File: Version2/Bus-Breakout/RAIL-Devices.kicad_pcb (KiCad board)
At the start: 2 copper layers, 99.8 x 19.5 mm, 33 parts, among them J2 Conn_01x30_Pin, J5 Conn_02x30_Odd_Even, P1 Jumper4x1, P10 Jumper4x1, P11 Jumper4x1, P12 Jumper4x1, P13 Jumper4x1, P14 Jumper4x1, P15 Jumper4x1, P16 Jumper4x1, P17 Jumper4x1, P18 Jumper4x1, P19 Jumper4x1, P2 Jumper4x1, P20 Jumper4x1, P21 Jumper4x1, P22 Jumper4x1, P23 Jumper4x1, P24 Jumper4x1, P25 Jumper4x1, P26 Jumper4x1, P27 Jumper4x1, P28 Jumper4x1, P29 Jumper4x1, P3 Jumper4x1, P30 Jumper4x1, P4 Jumper4x1, P5 Jumper4x1, P6 Jumper4x1, P7 Jumper4x1, P8 Jumper4x1, P9 Jumper4x1

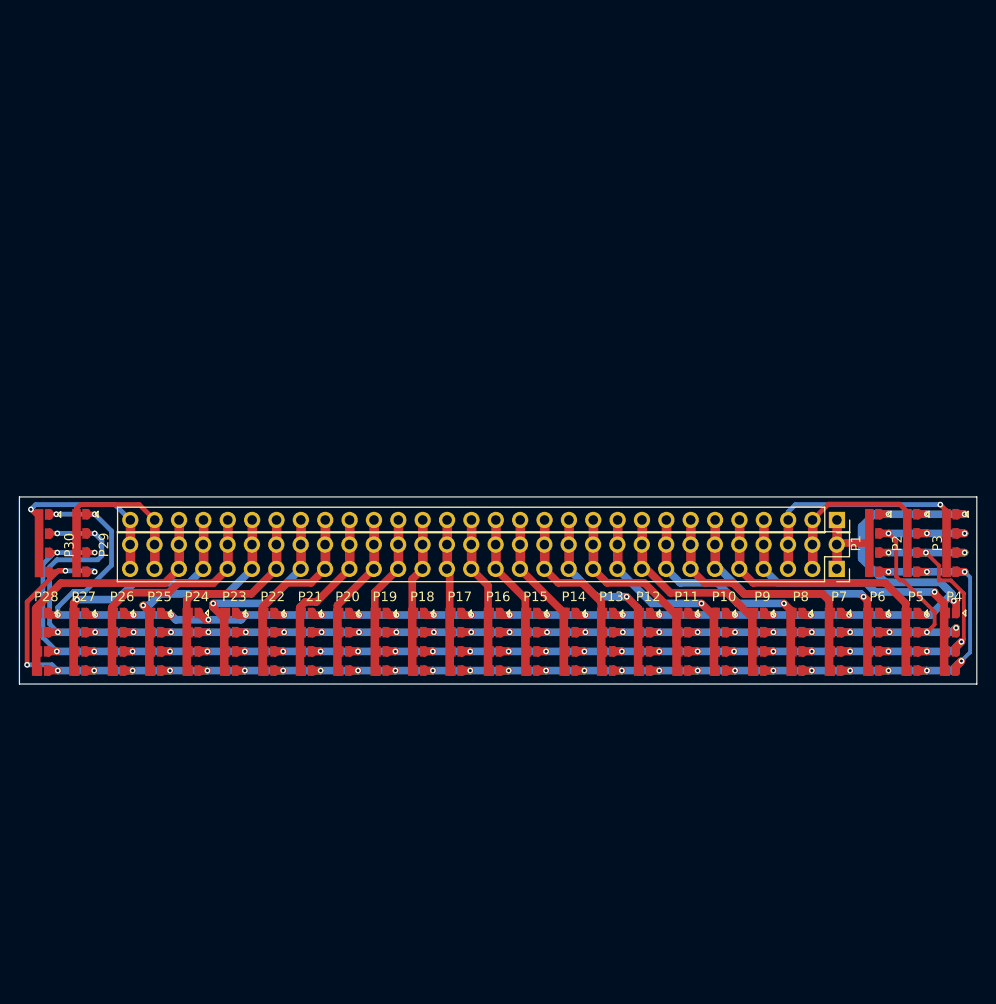
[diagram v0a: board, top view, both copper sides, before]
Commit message: updates.
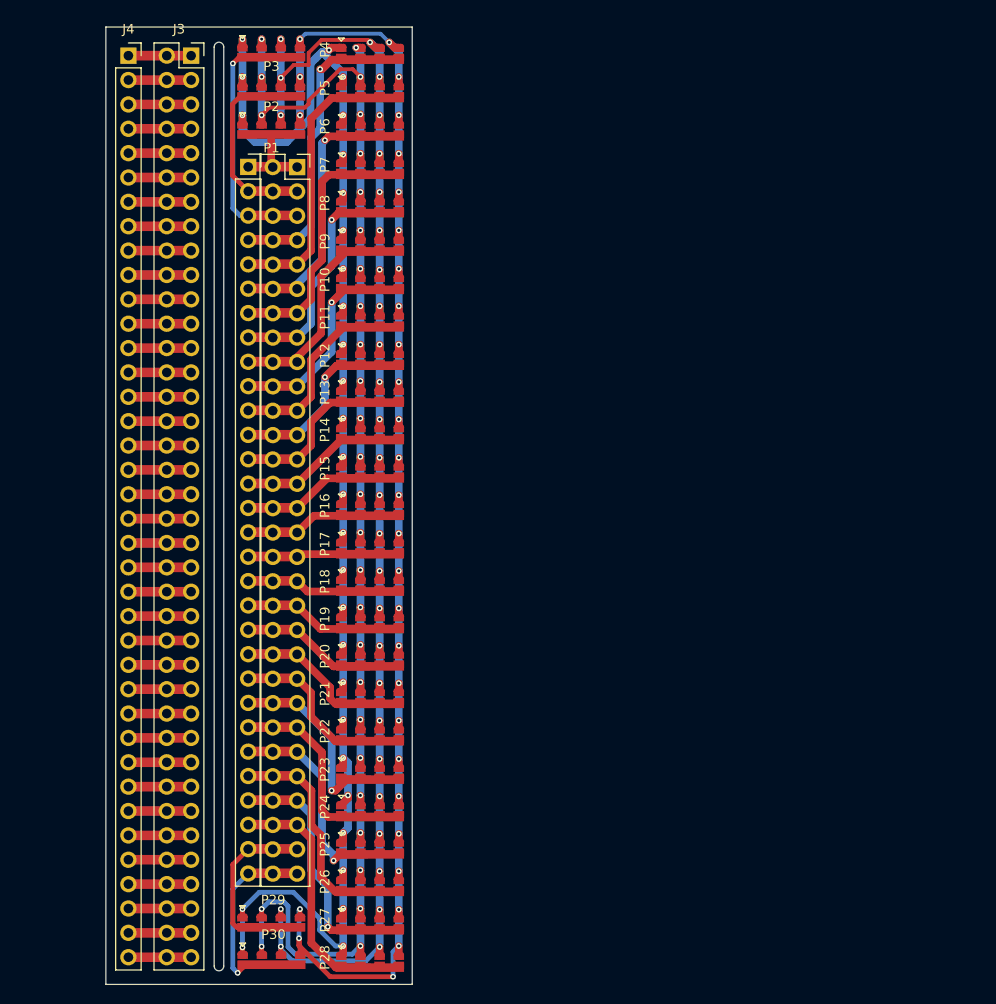
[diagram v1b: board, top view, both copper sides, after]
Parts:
- added J3: Conn_02x38_Odd_Even, Connector_PinSocket_2.54mm:PinSocket_2x38_P2.54mm_Vertical, F.Cu at (110.5, 44.9)
- added J4: Conn_01x38_Pin, Connector_PinSocket_2.54mm:PinSocket_1x38_P2.54mm_Vertical, F.Cu at (104.0, 44.9)
- moved P3 87.5 mm to (115.8, 45.1), turned to 90 degrees
- moved P4 85.3 mm to (126.1, 45.3), turned to 90 degrees
- moved P2 81.9 mm to (115.8, 49.1), turned to 90 degrees
- moved P5 79.7 mm to (126.1, 49.3), turned to 90 degrees
- moved P1 76.4 mm to (115.8, 53.1), turned to 90 degrees
- moved P6 74.0 mm to (126.1, 53.3), turned to 90 degrees
- moved J2 71.6 mm to (116.4, 56.5), turned to 0 degrees
- moved J5 70.1 mm to (121.5, 56.5), turned to 0 degrees
- moved P7 68.4 mm to (126.1, 57.3), turned to 90 degrees
- moved P8 62.7 mm to (126.1, 61.3), turned to 90 degrees
- moved P9 57.1 mm to (126.1, 65.3), turned to 90 degrees
- moved P30 51.5 mm to (115.9, 139.7), turned to 90 degrees
- moved P10 51.4 mm to (126.1, 69.3), turned to 90 degrees
- moved P28 48.8 mm to (126.1, 140.0), turned to 90 degrees
- moved P29 46.4 mm to (115.8, 135.8), turned to 90 degrees
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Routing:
- net /B9: track 0.00 -> 6.54 mm
- net /B8: track 0.00 -> 6.54 mm
- net /B7: track 0.00 -> 6.54 mm
- net /B6: track 0.00 -> 6.54 mm
- net /B5: track 0.00 -> 6.54 mm
- net /B4: track 0.00 -> 6.54 mm
- net /B38: track 0.00 -> 6.54 mm
- net /B37: track 0.00 -> 6.54 mm
- net /B36: track 0.00 -> 6.54 mm
- net /B35: track 0.00 -> 6.54 mm
- net /B34: track 0.00 -> 6.54 mm
- net /B33: track 0.00 -> 6.54 mm
- net /B32: track 0.00 -> 6.54 mm
- net /B31: track 0.00 -> 6.54 mm
- net /B30: track 0.00 -> 6.54 mm
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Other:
- board size 99.8 x 19.5 mm -> 31.9 x 99.8 mm
